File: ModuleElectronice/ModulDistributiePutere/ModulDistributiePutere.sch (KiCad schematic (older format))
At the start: 24 parts

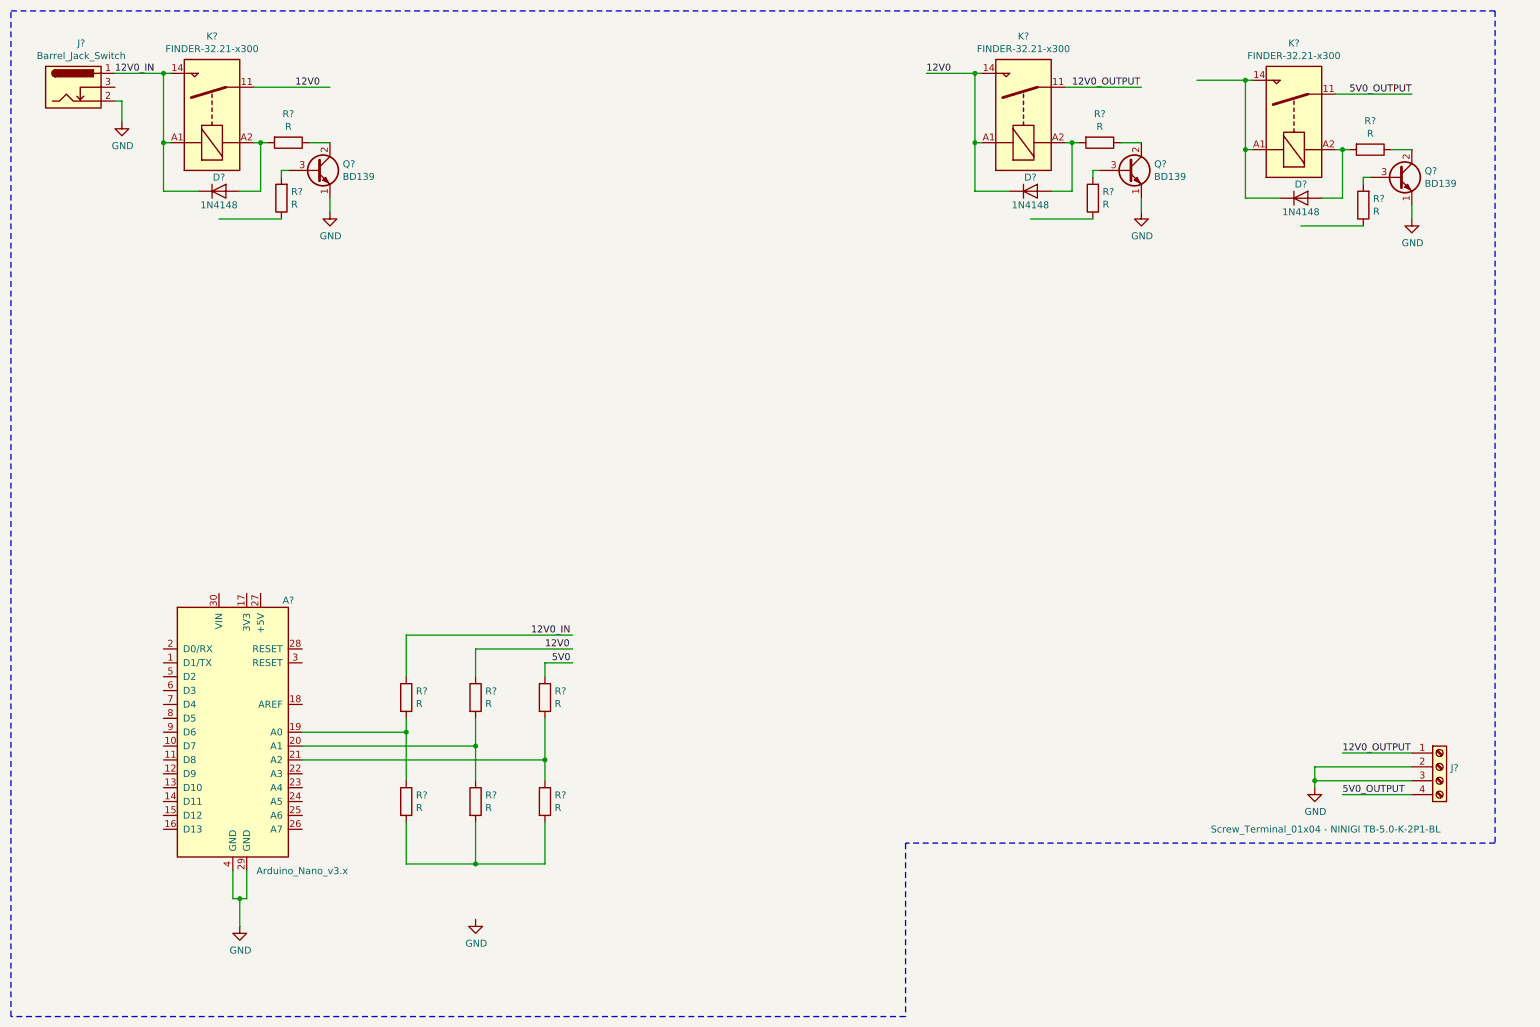
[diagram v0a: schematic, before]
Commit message: Updated files + Documentation April 7 - 2019
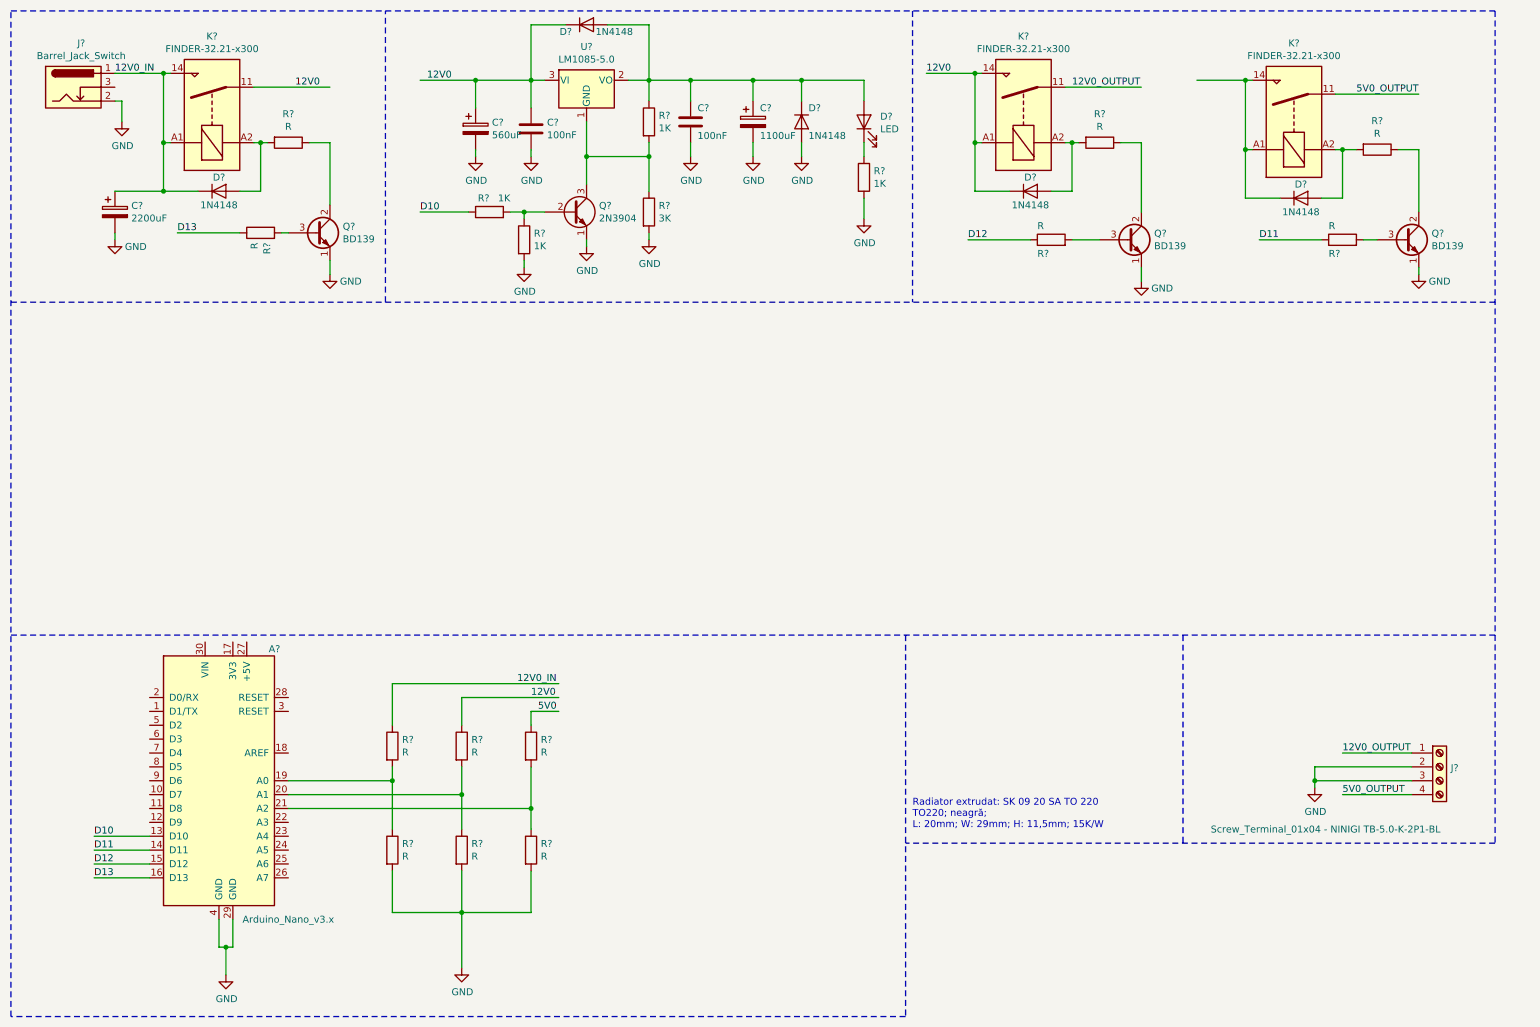
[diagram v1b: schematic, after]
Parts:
- added C?: 1100uF, symbol Device:CP
- added C?: 560uF, symbol Device:CP
- added C?: 2200uF, symbol Device:CP
- added C? (x2): 100nF, symbol Device:C
- added D? (x2): 1N4148, Diode_THT:D_DO-35_SOD27_P7.62mm_Horizontal, symbol Diode:1N4148
- added D?: LED, symbol Device:LED
- added Q?: 2N3904, Package_TO_SOT_THT:TO-92_Inline, symbol Transistor_BJT:2N3904
- added R?: 3K, symbol Device:R
- added R? (x4): 1K, symbol Device:R
- added U?: LM1085-5.0, symbol Regulator_Linear:LM1085-5.0
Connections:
- net labels added: D10, D11, D12, D13
- wire segments 81 -> 126
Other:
- note added: "Radiator extrudat: SK 09 20 SA TO 220\nTO220; neagră; \nL: 20mm; W: 29mm; H: 11,5mm; 15K/W"
- moved on the sheet: A?, Q?, R?
